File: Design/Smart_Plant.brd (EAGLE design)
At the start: 80 x 111.8 mm, 85 parts, among them IC1 NE555D, Q1 IRLML0100, Q3 2.5A/30V, Q4 MBT3904DW1T1, U10 ESP3212, U6 W25Q32FVSS, U7 FT231XS, U8 MCP73831, U9 AP2112K-3.3V, X2 MICROSD, Y3 26MHz

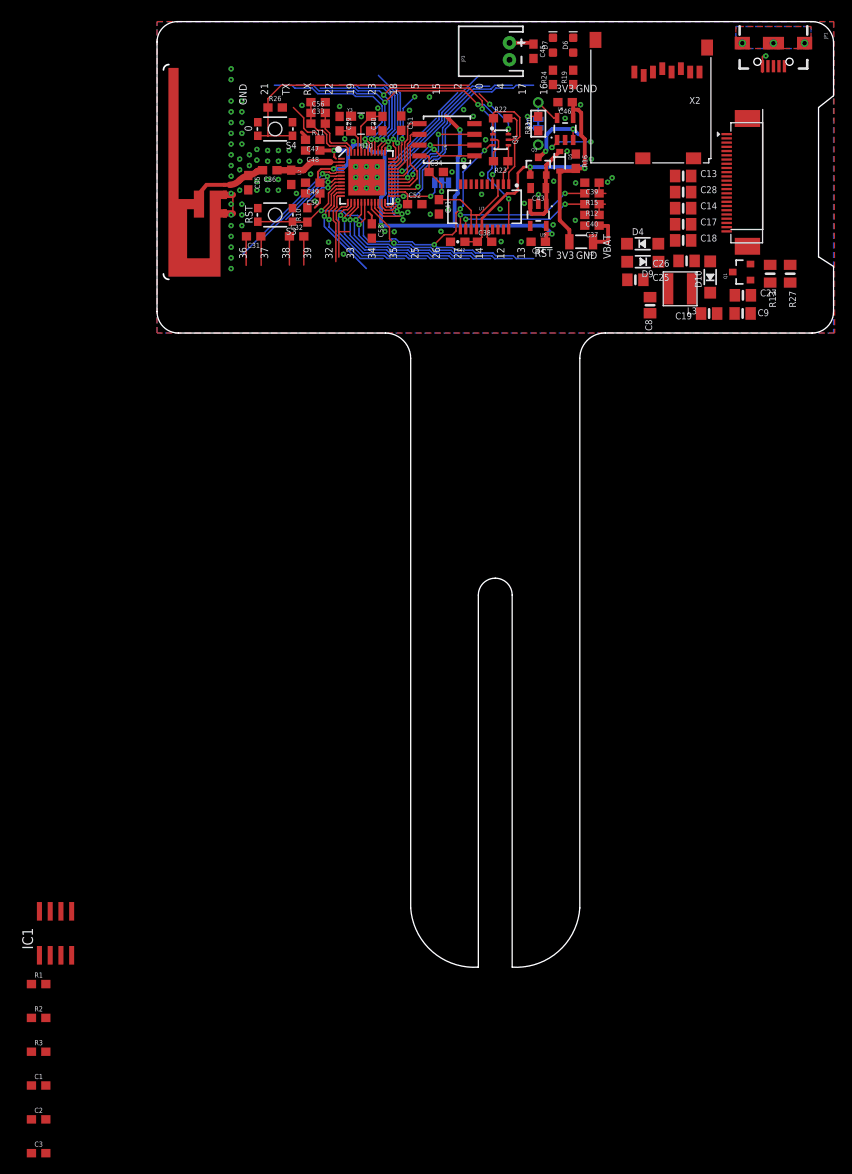
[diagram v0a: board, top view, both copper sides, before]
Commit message: Updated design files for Smart_Plant
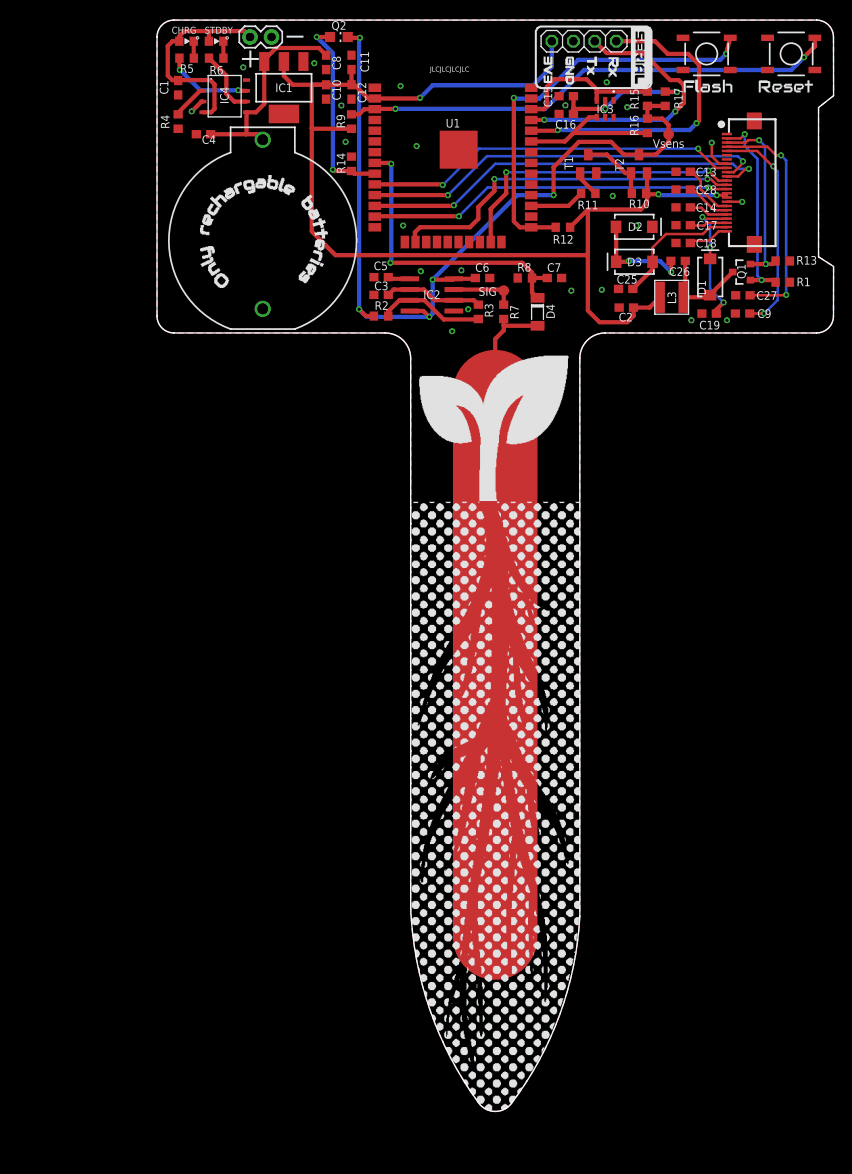
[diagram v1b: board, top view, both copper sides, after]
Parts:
- removed C29, C30: 10pF, SparkFun-Capacitors:0603
- removed C31, C32: 270pF, esp32-thing-temp:0603
- removed C33: 10nF, SparkFun-Capacitors:0603
- removed C34, C37, C38, C41, C48, C49, C51, C53: 0.1uF, SparkFun-Capacitors:0603
- removed C35: 2.4pF, esp32-thing-temp:0603
- removed C36: 5.6pF, esp32-thing-temp:0603
- removed C39, C40: 47pF, SparkFun-Capacitors:0603
- removed C42: 4.7uF, SparkFun-Capacitors:0603-CAP
- removed C43: 1.0uF, SparkFun-Capacitors:0805
- removed C44: 2.2uF, SparkFun-Capacitors:0603
- removed C45, C46: 4.7uF, SparkFun-Capacitors:0603
- removed C47: 100pF, SparkFun-Capacitors:0603
- removed C50: 10uF, SparkFun-Capacitors:0603
- removed C52: 1.0uF, SparkFun-Capacitors:0603
- removed C56: 3.0nF, esp32-thing-temp:0603
- removed D10, D9: MBR0530, microbuilder:SOD-123
- removed D5: BAT20J, SparkFun-DiscreteSemi:SOD-323
- removed D6: Yellow, SparkFun-LED:LED-0603
- removed D7: Green, SparkFun-LED:LED-0603
- removed E2: ANTENNA, esp32-thing-temp:TRACE_ANTENNA_2.4GHZ_25.7MM_TUNED
- removed EINK1: EINK_24PIN_290IN, microbuilder:EINK_290IN
- removed F2: 500mA, SparkFun-PowerIC:PTC-1206
- removed JP1: (no value), SparkFun-Connectors:USB-B-MICRO-SMD_V03
- removed JP3: LiPo, SparkFun-Connectors:JST-2-PTH
- removed L2: 2.7nH, SparkFun-Passives:0603
- removed Q3: 2.5A/30V, SparkFun-DiscreteSemi:SOT23-3
- removed Q4: MBT3904DW1T1, esp32-thing-temp:SC70-6
- removed R19, R24: 1K, SparkFun-Resistors:0603
- removed R20: 2.0k, SparkFun-Resistors:0603
- removed R21: DNP, SparkFun-Passives:1/6W-RES
- removed R22, R23, R26: 10k, SparkFun-Resistors:0603
- removed R27: DNP, microbuilder:0805_10MGAP
- removed S3: RESET, SparkFun-Electromechanical:TACTILE_SWITCH_SMD_4.6X2.8MM
- removed S4: BTN-0, SparkFun-Electromechanical:TACTILE_SWITCH_SMD_4.6X2.8MM
- removed SJ4: (no value), SparkFun-Passives:PAD-JUMPER-3-2OF3_NC_BY_TRACE_YES_SILK_FULL_BOX
- removed SJ5: JUMPER-PAD-2-NC_BY_TRACE, SparkFun-Passives:PAD-JUMPER-2-NC_BY_TRACE_YES_SILK
- removed U10: ESP3212, esp32-thing-temp:QFN48-0.4MM
- removed U6: W25Q32FVSS, SparkFun-DigitalIC:SOIC-8
- removed U7: FT231XS, SparkFun-DigitalIC:SSOP20_L
- removed U8: MCP73831, SparkFun-PowerIC:SOT23-5
- removed U9: AP2112K-3.3V, SparkFun-PowerIC:SOT23-5
- removed X2: MICROSD, microbuilder:MICROSD
- removed Y3: 26MHz, things:CRYSTAL-SMD-3.2X2.5
- added BT1: (no value), SparkFun-Batteries:BATTCOM_20MM_PTH
- added C10, C16, C4: 10uF, rcl:C0603
- added C11, C6: 100nF, rcl:C0603
- added C12: 22uF, rcl:C0603
- added C15: 0.1uF, rcl:C0603
- added C5: 10nF, rcl:C0603
- added C7: 1uF, rcl:C0603
- added D1, D2, D3: SS14, SparkFun-DiscreteSemi:SMA-DIODE
- added FPC: E-PAPER-FPC, SpaceDIY_connectors:FPC-05FB-24PH20
- added IC2: TLC555CDR, linear:SO08
- added IC3: AHT20, SamacSys_Parts:AHT20
- added IC4: TP4056, TP4056:SOT23-8
- added J1: (no value), SparkFun-Connectors:1X02
- added J3: (no value), pinhead:1X04
- added LED1: Red, SpaceDIY_semiconductors:LED_0603
- added LED2: Green, SpaceDIY_semiconductors:LED_0603
- added Q2: ALS-PT19-315C, SparkFun-DiscreteSemi:PT17-21C-L41-TR8
- added R14, R7: 10k, rcl:R0603
- added R17: 220, rcl:R0603
- added R4: 33k, rcl:R0603
- added R5: 1K, rcl:R0603
- added R6: 1k, rcl:R0603
- added R8: 1M, rcl:R0603
- added R9: 10K, rcl:R0603
- added S1: Flash, SpaceDIY_electromechanical:TACTILE_SWITCH_SMD_5.2MM
- added S2: Reset, SpaceDIY_electromechanical:TACTILE_SWITCH_SMD_5.2MM
- added T1: MMBT2222A, JLC PCB Basic Parts_loc:SOT23
- added T2: LBSS84LT1G, JLC PCB Basic Parts_loc:SOT23
- added TP1, TP2: TPB1,27, testpad:B1,27
- added U1: ESP-32S, esp32:ESP-32S
- C1: value 0.1uF -> 10uF; device SparkFun-Capacitors:0603 -> rcl:C0603
- C13, C14, C17, C18, C19, C25, C27, C28, C9: device microbuilder:0805-NO -> rcl:C0603
- C2: value 0.1uF -> 4.7uF; device SparkFun-Capacitors:0603 -> rcl:C0603
- C26: value 4.7uF/25V -> 4.7uF; device microbuilder:0805-NO -> rcl:C0603
- C3: value 0.1uF -> 0.47nF; device SparkFun-Capacitors:0603 -> rcl:C0603
- C8: value 10uF/10V+ -> 10uF; device microbuilder:0805-NO -> rcl:C0603
- D4: value MBR0530 -> LL4148; device microbuilder:SOD-123 -> SpaceDIY_semiconductors:LL-34
- IC1: value NE555D -> AMS1117-3.3; device linear:SO08 -> SparkFun-IC-Power:SOT223
- R1, R12, R15: value 27 -> 10k; device SparkFun-Resistors:0603 -> rcl:R0603
- R10, R16: device SparkFun-Resistors:0603 -> rcl:R0603
- R11: value 20k -> 1k; device SparkFun-Resistors:0603 -> rcl:R0603
- R13: value 0.47ohm -> 0.47; device microbuilder:0805_10MGAP -> rcl:R0603
- R2: value 27 -> 330R; device SparkFun-Resistors:0603 -> rcl:R0603
- R3: value 27 -> 1.5k; device SparkFun-Resistors:0603 -> rcl:R0603
- moved R1 121.0 mm to (74.0, 6.00)
- moved C1 119.1 mm to (2.50, 29.0), turned to 270 degrees
- moved C2 118.5 mm to (55.5, 3.00), turned to 180 degrees
- moved C3 109.3 mm to (26.5, 4.50), turned to 180 degrees
- moved IC1 103.6 mm to (15.0, 29.0), turned to 180 degrees
- moved R3 101.8 mm to (38.0, 2.50), turned to 90 degrees
- moved R2 92.4 mm to (26.5, 2.00)
- moved C8 47.9 mm to (20.0, 32.0), turned to 270 degrees
- moved R10 39.3 mm to (57.0, 16.5), turned to 180 degrees
- moved R11 33.0 mm to (51.0, 16.5), turned to 0 degrees
- moved D4 14.8 mm to (45.0, 2.50), turned to 270 degrees
- moved R15 13.0 mm to (58.0, 27.7), turned to 90 degrees
- moved R16 9.45 mm to (58.0, 24.5)
- moved R12 4.39 mm to (48.0, 12.5)
- moved R13 2.12 mm to (74.0, 8.51), turned to 0 degrees
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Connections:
- removed net 0: Q4.6, R26.1, S4.3, S4.4, U10.23
- removed net 12: U10.18
- removed net 19: U10.38
- removed net 21: U10.42
- removed net 22: U10.39
- removed net 25: U10.14
- removed net 26: U10.15
- removed net 27: U10.16
- removed net 3.3V_F: C41.1, U7.13, U7.14, U7.3
- removed net 32: U10.12
- removed net 33: U10.13
- removed net 34: U10.10
- removed net 35: U10.11
- removed net 36: C31.2, U10.5
- removed net 37: C31.1, U10.6
- removed net 38: C32.1, U10.7
- removed net 39: C32.2, U10.8
- removed net 3V3: C44.1, C47.1, C48.1, C49.1, C50.1, C51.1, C53.1, C8.2, EINK1.15, EINK1.16, L3.P$2, R10.2, R24.1, R26.2, SJ4.3, U10.1, U10.19, U10.3, U10.37, U10.4, U10.43, U10.46, U9.5, X2.4
- removed net CAP_10N1: C33.2, C56.1, R11.2, U10.48
- removed net CHIP_PU: Q4.3, R10.1, S3.3, S3.4, U10.9
- removed net D+: C39.1, JP1.D+, R15.1
- removed net D-: C40.1, JP1.D-, R12.1
- removed net DTR: Q4.1, R22.1, U7.1
- removed net FLASH_SCK: U10.31, U6.6
- removed net FLASH_SCS: U10.30, U6.1
- removed net FLASH_SDI: U10.33, U6.5
- removed net FLASH_SDO: U10.32, U6.2
- removed net FLASH_SHD: U10.28, U6.7
- removed net FLASH_SWP: U10.29, U6.3
- removed net FLASH_VDD: C52.1, SJ4.1, U10.26
- removed net LNA_IN1: C36.1, L2.1, U10.2
- removed net MISO_SD: U10.22, X2.7
- removed net MOSI_SD: U10.21, X2.3
- removed net N$19: D6.A, R19.2
- removed net N$20: D6.C, U8.1
- removed net N$21: R21.2, SJ5.2, U8.5
- removed net N$22: R20.2, SJ5.1
- removed net N$23: Q4.5, R22.2
- removed net N$24: Q4.2, R23.2
- removed net N$25: C29.2, U10.45, Y3.1
- removed net N$26: C30.2, U10.44, Y3.3
- removed net N$27: D7.A, R24.2
- removed net N$30: C56.2, R11.1, U10.47
- removed net RTS: Q4.4, R23.1, U7.2
- removed net SCLK_SD: U10.17, X2.5
- removed net SDCS_SD: U10.20, X2.2
- removed net SHIELD: JP1.SHIELD1, JP1.SHIELD2, JP1.SHIELD3
- removed net TRACE_ANT1: C35.1, C36.2, E2.ANT
- removed net TSCL: EINK1.6
- removed net TSDA: EINK1.7
- removed net U0RXD: U10.40, U7.20
- removed net U0TXD: U10.41, U7.4
- removed net V+: IC1.8
- removed net VUSB-RAW: C37.1, F2.1, JP1.VBUS
- removed net V_BATT: C45.1, JP3.2, Q3.3, U8.3
- removed net V_USB: C38.1, C42.1, C46.1, D5.A, F2.2, Q3.1, R16.2, R19.1, U7.15, U8.4
- new net 3.3V: C10.1, C11.1, C12.1, C2.1, FPC.15, FPC.16, IC1.2, J3.1, L3.P$2, R10.1, R12.1, R9.2, T2.2, U1.2
- new net IO0: R12.2, S1.3, U1.25
- new net LIGHT: Q2.E, R14.1, U1.9
- new net MOISTURE: C7.1, D4.C, R8.1, U1.8
- new net N$1: IC4.2, R4.2
- new net N$10: C15.1, C16.1, IC3.2, R17.2
- new net N$2: IC4.6, R6.2
- new net N$3: LED1.C, R5.1
- new net N$4: LED2.C, R6.1
- new net N$7: IC2.7, R2.2, R3.1
- new net N$8: C5.2, IC2.5
- new net N$9: R10.2, T1.3, T2.1
- new net OUT: IC2.3, R7.2, TP1.TP
- new net PROBE: D4.A, R7.1
- new net RST: R9.1, S2.3, U1.3
- new net RX: J3.4, U1.34
- new net SCL: IC3.3, R15.2, U1.36
- new net SDA: IC3.4, R16.2, U1.33
- new net SENS: R11.1, U1.27
- new net TX: J3.3, U1.35
- new net VBAT: BT1.1, C4.1, C8.1, IC1.3, IC4.5
- new net VSENS: C6.1, IC2.4, IC2.8, Q2.C, R15.1, R16.1, R17.1, R2.1, T2.3, TP2.TP
- net BUSY: now also FPC.9, U1.10; no longer EINK1.9, U10.24
- net DC: now also FPC.11, U1.12; no longer EINK1.11, U10.27
- net DISPCS: now also FPC.12, U1.23; no longer EINK1.12, U10.34
- net GDR: now also FPC.2, R1.1; no longer EINK1.2
- net GND: now also BT1.2, C1.2, C10.2, C11.2, C12.2, C15.2, C16.2, C2.2, C3.2, C4.2, C5.1, C6.2, C7.2, C8.2, D2.C, FPC.17, FPC.8, IC2.1, IC3.5, IC4.3, IC4.8, J1.2, J3.2, R1.2, R14.2, R4.1, R8.2, S1.1, S2.1, T1.2, U1.1, U1.15, U1.38, U1.GND; no longer C29.1, C30.1, C33.1, C34.2, C35.2, C37.2, C38.2, C39.2, C40.2, C41.2, C42.2, C43.2, C44.2, C45.2, C46.2, C47.2, C48.2, C49.2, C50.2, C51.2, C52.2, C53.2, C8.1, D4.C, D7.C, E2.GND, E2.GND2, EINK1.17, EINK1.8, JP1.GND, JP3.1, L2.2, R16.1, R20.1, R21.1, R27.2, S3.1, S3.2, S4.1, S4.2, U10.EP, U6.4, U7.16, U7.6, U8.2, U9.2, X2.6, X2.MT1, X2.MT2, Y3.2, Y3.4
- net MOSI: now also FPC.14, U1.13; no longer EINK1.14, U10.36
- net N$11: now also FPC.5; no longer EINK1.5
- net N$12: now also FPC.18; no longer EINK1.18
- net N$13: now also FPC.20; no longer EINK1.20
- net N$14: now also FPC.22; no longer EINK1.22
- net N$15: now also FPC.24; no longer EINK1.24
- net N$16: now also D2.A, D3.C; no longer D4.A, D9.C
- net N$17: now also D1.A; no longer D10.A
- net N$18: now also R11.2, T1.1; no longer R15.2, U7.11
- net N$31: now also FPC.4; no longer EINK1.4
- net N$32: now also FPC.19; no longer EINK1.19
- net N$5: now also C3.1, IC2.2, IC2.6, R3.2; no longer C34.1, SJ4.2, U6.8
- net N$6: now also IC4.7, R5.2; no longer R12.2, U7.12
- net RESE: now also FPC.3; no longer EINK1.3, R27.1
- net RESET: now also FPC.10, U1.11; no longer EINK1.10, U10.25
- net SCLK: now also FPC.13, U1.16; no longer EINK1.13, U10.35
- net VGH: now also D1.C, FPC.21; no longer D10.C, EINK1.21
- net VGL: now also D3.A, FPC.23; no longer D9.A, EINK1.23
- net VIN: now also C1.1, IC4.1, IC4.4, J1.1, LED1.A, LED2.A; no longer C43.1, D5.C, Q3.2, U9.1, U9.3
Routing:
- net 3.3V: track 0.00 -> 146.4 mm, vias 0 -> 3
- net VSENS: track 0.00 -> 102.9 mm, vias 0 -> 5
- net PROBE: track 0.00 -> 77.6 mm
- net 3V3: track 74.1 -> 0.00 mm, vias 8 -> 0
- net 0: track 62.2 -> 0.00 mm, vias 3 -> 0
- net RST: track 0.00 -> 59.1 mm, vias 0 -> 2
- net CHIP_PU: track 56.5 -> 0.00 mm, vias 4 -> 0
- net IO0: track 0.00 -> 49.2 mm, vias 0 -> 2
- net U0RXD: track 45.4 -> 0.00 mm, vias 4 -> 0
- net V_USB: track 43.1 -> 0.00 mm, vias 2 -> 0
- net U0TXD: track 41.0 -> 0.00 mm, vias 4 -> 0
- net RX: track 0.00 -> 37.9 mm, vias 0 -> 2
- net MOISTURE: track 0.00 -> 36.0 mm, vias 0 -> 2
- net TX: track 0.00 -> 33.7 mm, vias 0 -> 2
- net SCLK: track 10.2 -> 42.6 mm, vias 1 -> 2
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- removed copper zone on layer 1, net SHIELD
- removed copper zone on layer 16, net SHIELD
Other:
- board size 80 x 111.8 mm -> 80 x 129.1 mm
- board text added: "CHRG"
- board text added: "JLCJLCJLCJLC"
- board text added: "SIG"
- board text added: "STDBY"
- board text added: "Vsens"
- board text removed: "!RST!"
- board text removed: "0"
- board text removed: "12"
- board text removed: "13"
- board text removed: "14"
- board text removed: "15"
- board text removed: "16"
- board text removed: "17"
- board text removed: "18"
- board text removed: "19"
- board text removed: "2"
- board text removed: "21"
- board text removed: "22"
- board text removed: "23"
- board text removed: "25"
- board text removed: "26"
- board text removed: "27"
- board text removed: "32"
- board text removed: "33"
- board text removed: "34"
- board text removed: "35"
- board text removed: "36"
- board text removed: "37"
- board text removed: "38"
- board text removed: "39"
- board text removed: "3V3"
- board text removed: "4"
- board text removed: "5"
- board text removed: "Adafruit Industries"
- board text removed: "CHG PROG"
- board text removed: "E-Ink Display"
- board text removed: "FLASH VCC"
- board text removed: "GND"
- board text removed: "IC"
- board text removed: "RST"
- board text removed: "RX"
- board text removed: "RXI"
- board text removed: "TX"
- board text removed: "TXO"
- board text removed: "VBAT"
- board text removed: "VUSB"

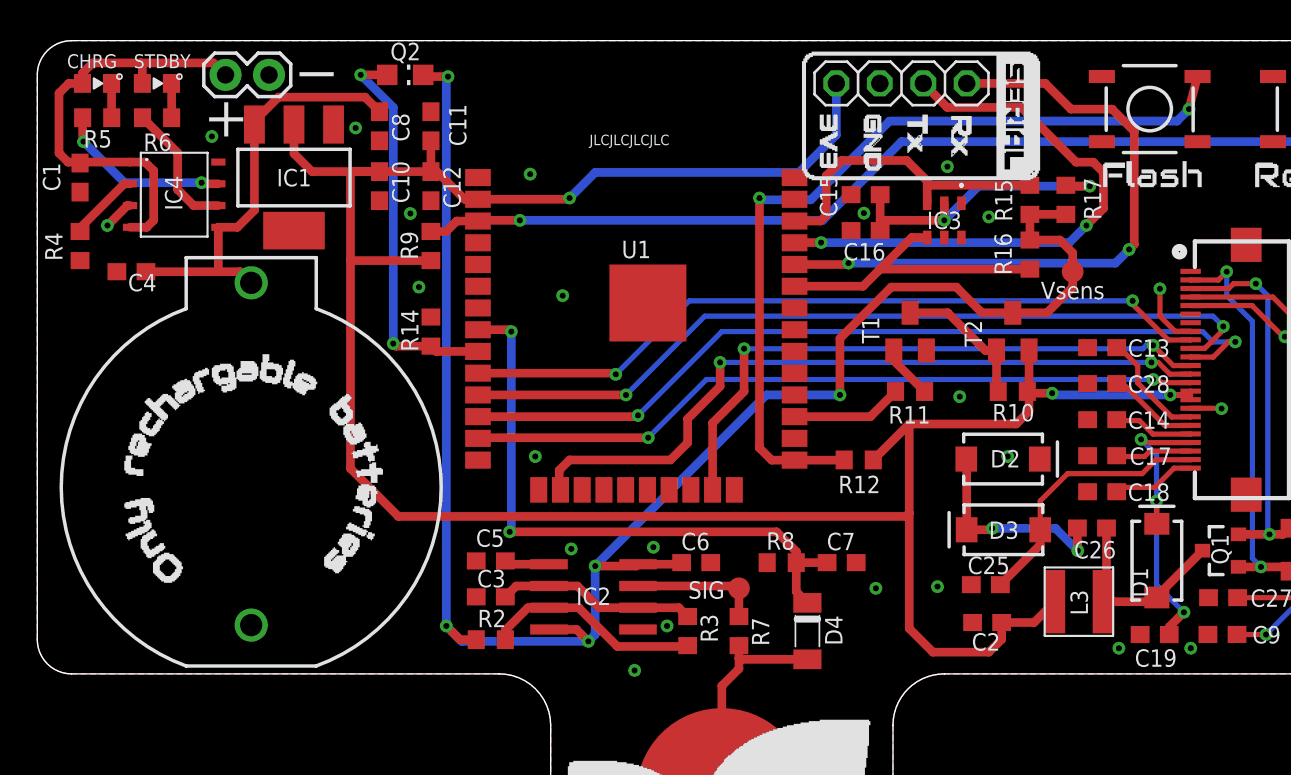
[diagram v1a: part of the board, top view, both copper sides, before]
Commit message: Update design files
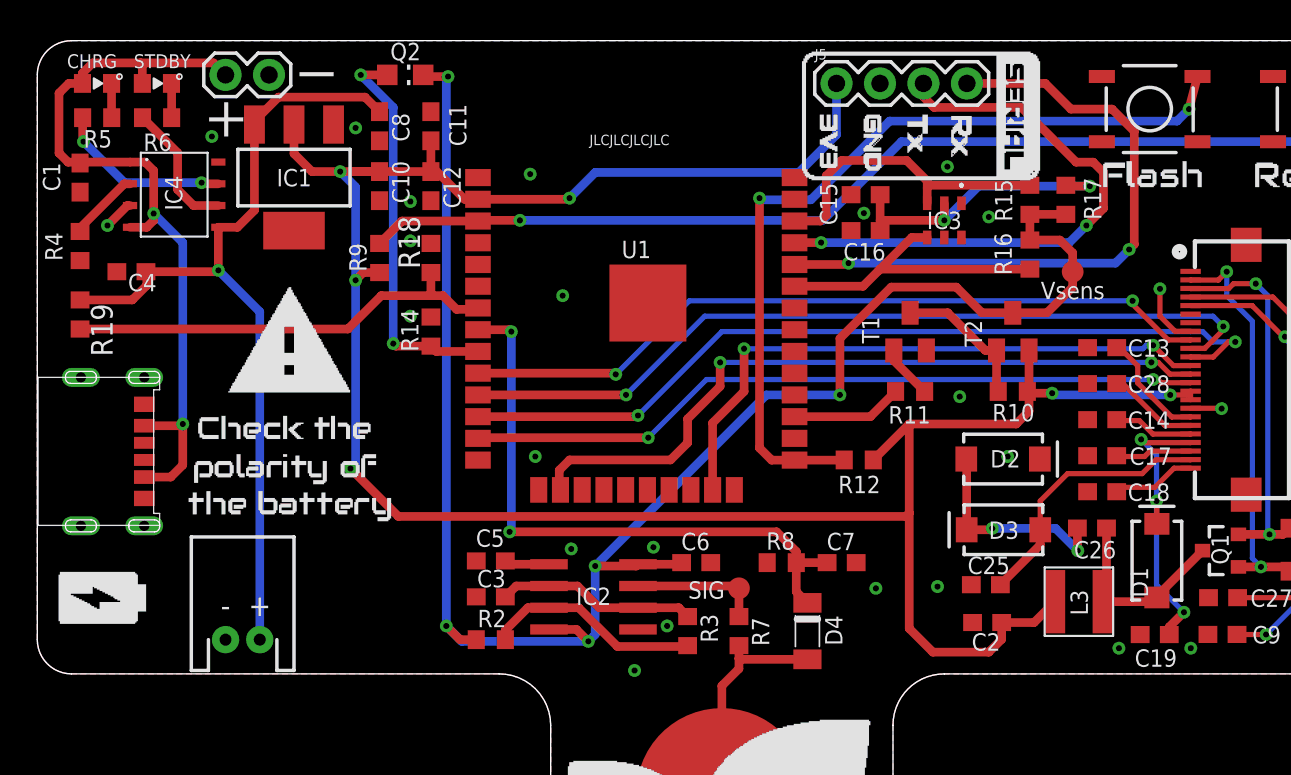
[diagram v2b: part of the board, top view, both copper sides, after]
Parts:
- removed BT1: (no value), SparkFun-Batteries:BATTCOM_20MM_PTH
- removed J3: (no value), pinhead:1X04
- added J2: USBC-6P, SpaceDIY_connectors:USCX-06FX-XXMX-01
- added J4: (no value), SparkFun-Connectors:JST-2-PTH-NS
- added J5: (no value), SparkFun-Connectors:1X04
- added R18: 240k, rcl:R0603
- added R19: 1M, rcl:R0603
- R4: value 33k -> 1.2k
- moved R9 3.08 mm to (20.0, 24.3)
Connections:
- new net BATTERY: R18.1, R19.2, U1.7
- net 3.3V: now also J5.1; no longer J3.1
- net GND: now also J2.GND1, J2.GND2, J4.1, J5.2, R18.2; no longer BT1.2, J3.2
- net RX: now also J5.4; no longer J3.4
- net TX: now also J5.3; no longer J3.3
- net VBAT: now also J4.2, R19.1; no longer BT1.1
- net VIN: now also J2.VBUS1, J2.VBUS2
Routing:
- net BATTERY: track 0.00 -> 25.8 mm
- net VBAT: track 25.0 -> 50.4 mm, vias 0 -> 1
- net VIN: track 26.7 -> 46.9 mm, vias 0 -> 2
- net 3.3V: track 146.4 -> 142.9 mm, vias 3 -> 6
- net RST: track 59.1 -> 62.4 mm
- net TX: track 33.7 -> 34.2 mm
- net GND: vias 23 -> 24
